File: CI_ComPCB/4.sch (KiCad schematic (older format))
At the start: 12 parts, among them IC301 TPS63020DSJR, J301 Connector_Conn_01x02_Male, J302 Connector_Conn_01x02_Male

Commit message: V1.1 Rough
Almost complete
needs silk screen annotations then will be ready to have printed
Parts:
- D301: symbol SamacSys_Parts:SS34 -> CI_ComPCB-rescue:SS34-SamacSys_Parts
- IC301: symbol SamacSys_Parts:TPS63020DSJR -> CI_ComPCB-rescue:TPS63020DSJR-SamacSys_Parts
- J301, J302: symbol CI_ComPCB-cache:Connector_Conn_01x02_Male -> CI_ComPCB-rescue:Connector_Conn_01x02_Male-CI_ComPCB-cache
- L301: symbol SamacSys_Parts:SPM4012T-1R0M-LR -> CI_ComPCB-rescue:SPM4012T-1R0M-LR-SamacSys_Parts
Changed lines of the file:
@@
 	6570 3680 6820 3680
 $Comp
-L SamacSys_Parts:TPS63020DSJR IC?
+L CI_ComPCB-rescue:TPS63020DSJR-SamacSys_Parts IC?
 U 1 1 61A532F4
 P 5770 4280
@@
 Buck_Converter_OUT
 $Comp
-L CI_ComPCB-cache:Connector_Conn_01x02_Male J301
+L CI_ComPCB-rescue:Connector_Conn_01x02_Male-CI_ComPCB-cache J301
 U 1 1 61294C10
 P 3410 3380
+AR Path="/61294C10" Ref="J301"  Part="1"
+AR Path="/61A31654/61294C10" Ref="J301"  Part="1"
 F 0 "J301" V 3472 3424 50  0000 L CNN
 F 1 "Connector_Conn_01x02_Male" V 3563 3424 50  0000 L CNN
@@
 $EndComp
 $Comp
-L CI_ComPCB-cache:Connector_Conn_01x02_Male J302
+L CI_ComPCB-rescue:Connector_Conn_01x02_Male-CI_ComPCB-cache J302
 U 1 1 61298A1D
 P 7470 3300
+AR Path="/61298A1D" Ref="J302"  Part="1"
+AR Path="/61A31654/61298A1D" Ref="J302"  Part="1"
 F 0 "J302" V 7532 3344 50  0000 L CNN
 F 1 "Connector_Conn_01x02_Male" V 7623 3344 50  0000 L CNN
@@
 $EndComp
 $Comp
-L SamacSys_Parts:SS34 D301
+L CI_ComPCB-rescue:SS34-SamacSys_Parts D301
 U 1 1 612A7837
 P 3450 3580
@@
 	4150 3580 4140 3580
 $Comp
-L SamacSys_Parts:SPM4012T-1R0M-LR L301
+L CI_ComPCB-rescue:SPM4012T-1R0M-LR-SamacSys_Parts L301
 U 1 1 612BD9BA
 P 5180 2700

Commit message: V1.1 Changed Diode for reprint
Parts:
- D301: footprint SamacSys_Parts:DIOM8059X256N -> digikey-footprints:DO-214AC
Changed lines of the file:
@@
 F 0 "D301" H 3850 3847 50  0000 C CNN
 F 1 "SS34" H 3850 3756 50  0000 C CNN
-F 2 "SamacSys_Parts:DIOM8059X256N" H 3950 3730 50  0001 L CNN
+F 2 "digikey-footprints:DO-214AC" H 3950 3730 50  0001 L CNN
 F 3 "https://componentsearchengine.com/Datasheets/2/SS34.pdf" H 3950 3630 50  0001 L CNN
 F 4 "ON Semi SS34 SMT Schottky Diode, 40V 3A, 2-Pin DO-214AB" H 3950 3530 50  0001 L CNN "Description"

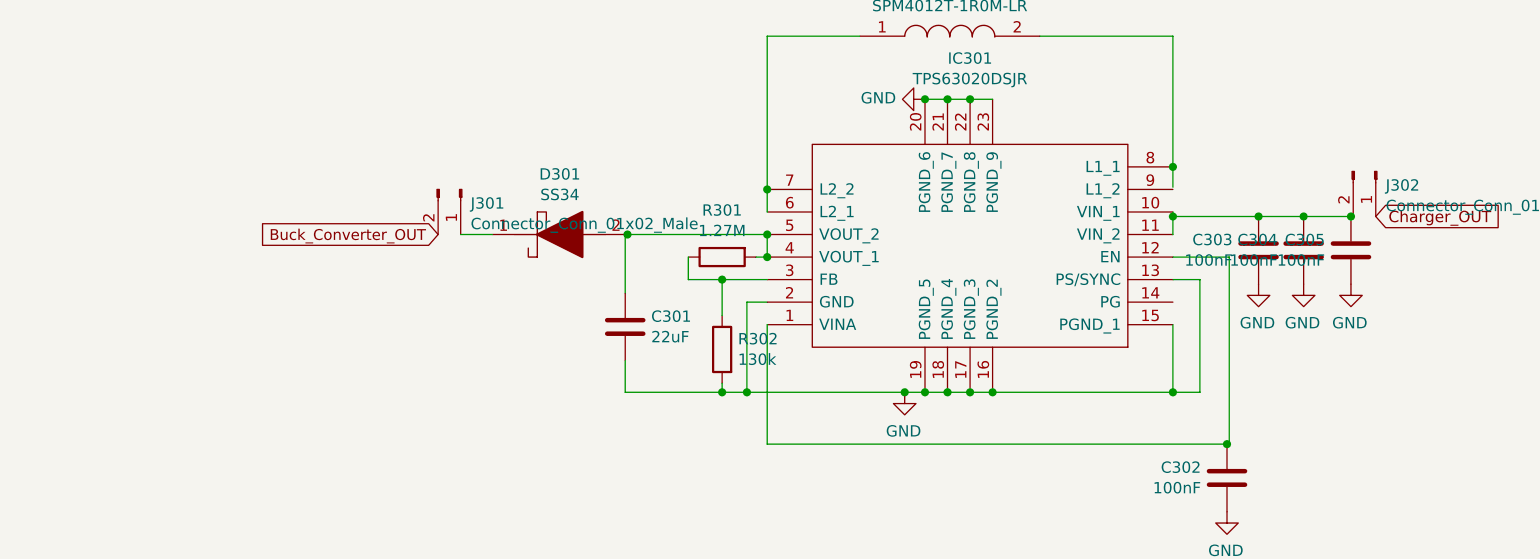
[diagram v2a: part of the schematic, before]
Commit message: converters debug
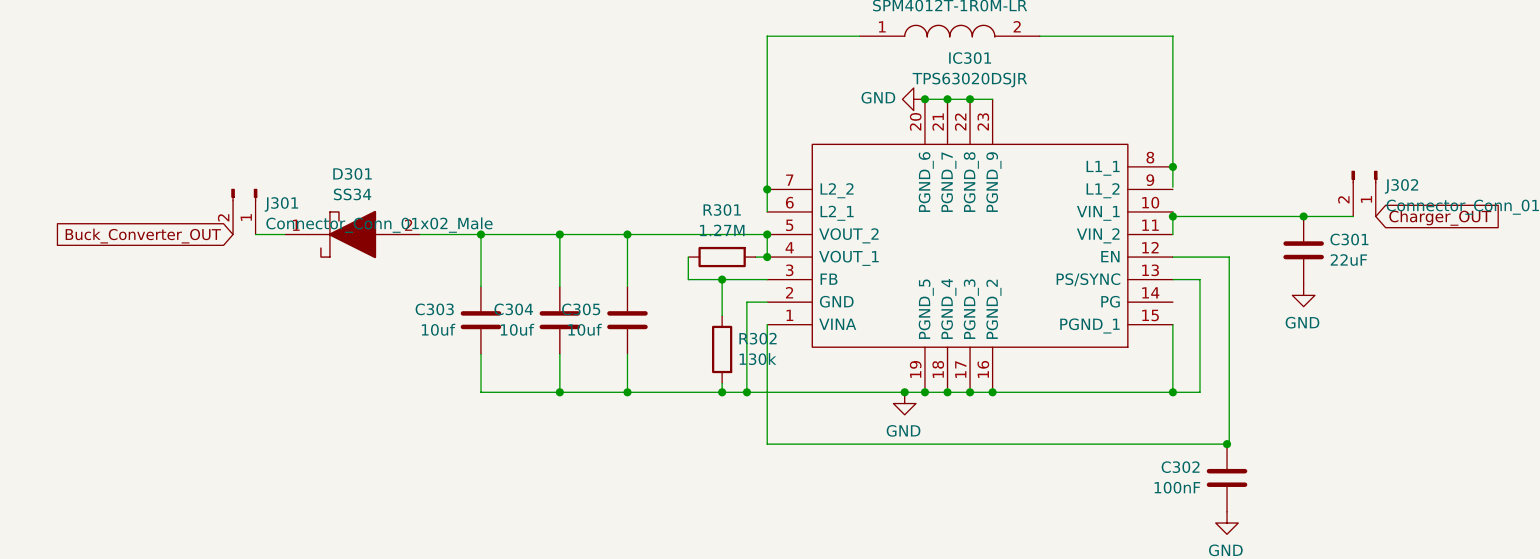
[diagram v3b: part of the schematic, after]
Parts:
- C303, C304, C305: value 100nF -> 10uf
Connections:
- net at IC301.10 (VIN_1), IC301.11 (VIN_2), J302.2 (Pin_2): now also C301.1; no longer C303.1, C304.1, C305.1
- net at D301.2, IC301.4 (VOUT_1), IC301.5 (VOUT_2)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: now also C303.1, C304.1, C305.1; no longer C301.1
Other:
- moved on the sheet: C301, C303, C304, C305, D301, J301
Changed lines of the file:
@@
 L Device:C C?
 U 1 1 61A53270
-P 4140 3990
+P 7150 3650
 AR Path="/61A53270" Ref="C?"  Part="1"
 AR Path="/61A31654/61A53270" Ref="C301"  Part="1"
-F 0 "C301" H 4025 4036 50  0000 R CNN
-F 1 "22uF" H 4025 3945 50  0000 R CNN
-F 2 "Capacitor_SMD:C_0805_2012Metric" H 4178 3840 50  0001 C CNN
-F 3 "~" H 4140 3990 50  0001 C CNN
-	1    4140 3990
-	-1   0    0    -1
-$EndComp
-Wire Wire Line
-	4770 3580 4150 3580
-Wire Wire Line
-	4140 3580 4140 3840
+F 0 "C301" H 7035 3696 50  0000 R CNN
+F 1 "22uF" H 7035 3605 50  0000 R CNN
+F 2 "Capacitor_SMD:C_0805_2012Metric" H 7188 3500 50  0001 C CNN
+F 3 "~" H 7150 3650 50  0001 C CNN
+	1    7150 3650
+	-1   0    0    -1
+$EndComp
 Wire Wire Line
 	5180 2700 4770 2700
@@
 	4570 4240 4570 4280
 Wire Wire Line
-	4570 4280 4140 4280
-Connection ~ 4570 4280
-Wire Wire Line
-	4140 4280 4140 4140
-Wire Wire Line
 	4770 4510 4770 3980
 Wire Wire Line
@@
 L Device:C C?
 U 1 1 61A532A2
-P 6950 3650
+P 3500 3960
 AR Path="/61A532A2" Ref="C?"  Part="1"
 AR Path="/61A31654/61A532A2" Ref="C303"  Part="1"
-F 0 "C303" H 7065 3696 50  0000 L CNN
-F 1 "100nF" H 7065 3605 50  0000 L CNN
-F 2 "Capacitor_SMD:C_0805_2012Metric" H 6988 3500 50  0001 C CNN
-F 3 "~" H 6950 3650 50  0001 C CNN
-	1    6950 3650
-	-1   0    0    -1
-$EndComp
-$Comp
-L power:GND #PWR?
-U 1 1 61A532A8
-P 6950 3800
-AR Path="/61A532A8" Ref="#PWR?"  Part="1"
-AR Path="/61A31654/61A532A8" Ref="#PWR0304"  Part="1"
-F 0 "#PWR0304" H 6950 3550 50  0001 C CNN
-F 1 "GND" H 6955 3627 50  0000 C CNN
-F 2 "" H 6950 3800 50  0001 C CNN
-F 3 "" H 6950 3800 50  0001 C CNN
-	1    6950 3800
-	-1   0    0    -1
-$EndComp
-Wire Wire Line
-	7370 3500 7360 3500
+F 0 "C303" H 3615 4006 50  0000 L CNN
+F 1 "10uf" H 3615 3915 50  0000 L CNN
+F 2 "Capacitor_SMD:C_0805_2012Metric" H 3538 3810 50  0001 C CNN
+F 3 "~" H 3500 3960 50  0001 C CNN
+	1    3500 3960
+	-1   0    0    -1
+$EndComp
 Text GLabel 7470 3500 2    50   Input ~ 0
 Charger_OUT
-Wire Wire Line
-	3410 3580 3550 3580
 Text Notes 7000 7110 0    50   ~ 0
 https://webench.ti.com/power-designer/switching-regulator/customize/6?noparams=0
@@
 L Device:C C?
 U 1 1 61A532B9
-P 7150 3650
+P 3850 3960
 AR Path="/61A532B9" Ref="C?"  Part="1"
 AR Path="/61A31654/61A532B9" Ref="C304"  Part="1"
-F 0 "C304" H 7265 3696 50  0000 L CNN
-F 1 "100nF" H 7265 3605 50  0000 L CNN
-F 2 "Capacitor_SMD:C_0805_2012Metric" H 7188 3500 50  0001 C CNN
-F 3 "~" H 7150 3650 50  0001 C CNN
-	1    7150 3650
+F 0 "C304" H 3965 4006 50  0000 L CNN
+F 1 "10uf" H 3965 3915 50  0000 L CNN
+F 2 "Capacitor_SMD:C_0805_2012Metric" H 3888 3810 50  0001 C CNN
+F 3 "~" H 3850 3960 50  0001 C CNN
+	1    3850 3960
 	-1   0    0    -1
 $EndComp
@@
 L Device:C C?
 U 1 1 61A532C5
-P 7360 3650
+P 4150 3960
 AR Path="/61A532C5" Ref="C?"  Part="1"
 AR Path="/61A31654/61A532C5" Ref="C305"  Part="1"
-F 0 "C305" H 7475 3696 50  0000 L CNN
-F 1 "100nF" H 7475 3605 50  0000 L CNN
-F 2 "Capacitor_SMD:C_0805_2012Metric" H 7398 3500 50  0001 C CNN
-F 3 "~" H 7360 3650 50  0001 C CNN
-	1    7360 3650
-	-1   0    0    -1
-$EndComp
-$Comp
-L power:GND #PWR?
-U 1 1 61A532CB
-P 7360 3800
-AR Path="/61A532CB" Ref="#PWR?"  Part="1"
-AR Path="/61A31654/61A532CB" Ref="#PWR0306"  Part="1"
-F 0 "#PWR0306" H 7360 3550 50  0001 C CNN
-F 1 "GND" H 7365 3627 50  0000 C CNN
-F 2 "" H 7360 3800 50  0001 C CNN
-F 3 "" H 7360 3800 50  0001 C CNN
-	1    7360 3800
-	-1   0    0    -1
-$EndComp
-Connection ~ 7150 3500
-Connection ~ 7360 3500
-Wire Wire Line
-	7360 3500 7150 3500
-Wire Wire Line
-	6950 3500 7150 3500
+F 0 "C305" H 4265 4006 50  0000 L CNN
+F 1 "10uf" H 4265 3915 50  0000 L CNN
+F 2 "Capacitor_SMD:C_0805_2012Metric" H 4188 3810 50  0001 C CNN
+F 3 "~" H 4150 3960 50  0001 C CNN
+	1    4150 3960
+	-1   0    0    -1
+$EndComp
 Connection ~ 6570 3280
 Connection ~ 5670 4280
@@
 Wire Wire Line
 	6570 3480 6570 3500
-Wire Wire Line
-	6950 3500 6570 3500
-Connection ~ 6950 3500
 Connection ~ 6570 3500
 Wire Wire Line
 	6570 3500 6570 3580
-Text GLabel 3310 3580 0    48   Input ~ 0
+Text GLabel 2400 3580 0    48   Input ~ 0
 Buck_Converter_OUT
 $Comp
 L CI_ComPCB-rescue:Connector_Conn_01x02_Male-CI_ComPCB-cache J301
 U 1 1 61294C10
-P 3410 3380
+P 2500 3380
 AR Path="/61294C10" Ref="J301"  Part="1"
 AR Path="/61A31654/61294C10" Ref="J301"  Part="1"
-F 0 "J301" V 3472 3424 50  0000 L CNN
-F 1 "Connector_Conn_01x02_Male" V 3563 3424 50  0000 L CNN
-F 2 "Connector_PinHeader_2.54mm:PinHeader_1x02_P2.54mm_Vertical" H 3410 3380 50  0001 C CNN
-F 3 "" H 3410 3380 50  0001 C CNN
-	1    3410 3380
+F 0 "J301" V 2562 3424 50  0000 L CNN
+F 1 "Connector_Conn_01x02_Male" V 2653 3424 50  0000 L CNN
+F 2 "Connector_PinHeader_2.54mm:PinHeader_1x02_P2.54mm_Vertical" H 2500 3380 50  0001 C CNN
+F 3 "" H 2500 3380 50  0001 C CNN
+	1    2500 3380
 	0    1    1    0
 $EndComp
@@
 	0    1    1    0
 $EndComp
-$Comp
-L CI_ComPCB-rescue:SS34-SamacSys_Parts D301
-U 1 1 612A7837
-P 3450 3580
-F 0 "D301" H 3850 3847 50  0000 C CNN
-F 1 "SS34" H 3850 3756 50  0000 C CNN
-F 2 "digikey-footprints:DO-214AC" H 3950 3730 50  0001 L CNN
-F 3 "https://componentsearchengine.com/Datasheets/2/SS34.pdf" H 3950 3630 50  0001 L CNN
-F 4 "ON Semi SS34 SMT Schottky Diode, 40V 3A, 2-Pin DO-214AB" H 3950 3530 50  0001 L CNN "Description"
-F 5 "2.56" H 3950 3430 50  0001 L CNN "Height"
-F 6 "512-SS34" H 3950 3330 50  0001 L CNN "Mouser Part Number"
-F 7 "https://www.mouser.co.uk/ProductDetail/ON-Semiconductor-Fairchild/SS34?qs=2ONuHmP%2FXzb3ub11UdFfdQ%3D%3D" H 3950 3230 50  0001 L CNN "Mouser Price/Stock"
-F 8 "ON Semiconductor" H 3950 3130 50  0001 L CNN "Manufacturer_Name"
-F 9 "SS34" H 3950 3030 50  0001 L CNN "Manufacturer_Part_Number"
-	1    3450 3580
-	1    0    0    -1
-$EndComp
-Connection ~ 4150 3580
-Wire Wire Line
-	4150 3580 4140 3580
 $Comp
 L CI_ComPCB-rescue:SPM4012T-1R0M-LR-SamacSys_Parts L301
@@
 Wire Wire Line
 	5980 2700 6570 2700
+Wire Wire Line
+	6570 3500 7150 3500
+Wire Wire Line
+	3500 4280 3500 4110
+Connection ~ 4570 4280
+Wire Wire Line
+	3850 4110 3850 4280
+Connection ~ 3850 4280
+Wire Wire Line
+	3850 4280 3500 4280
+Wire Wire Line
+	4570 4280 4150 4280
+Wire Wire Line
+	4150 4110 4150 4280
+Connection ~ 4150 4280
+Wire Wire Line
+	4150 4280 3850 4280
+Wire Wire Line
+	3500 3810 3500 3580
+Connection ~ 3500 3580
+Wire Wire Line
+	3850 3810 3850 3580
+Connection ~ 3850 3580
+Wire Wire Line
+	3850 3580 3500 3580
+Wire Wire Line
+	4770 3580 4150 3580
+Wire Wire Line
+	4150 3810 4150 3580
+Connection ~ 4150 3580
+Wire Wire Line
+	4150 3580 3850 3580
+Connection ~ 7150 3500
+Wire Wire Line
+	7150 3500 7370 3500
+Wire Wire Line
+	3230 3580 3500 3580
+$Comp
+L CI_ComPCB-rescue:SS34-SamacSys_Parts D301
+U 1 1 612A7837
+P 2530 3580
+F 0 "D301" H 2930 3847 50  0000 C CNN
+F 1 "SS34" H 2930 3756 50  0000 C CNN
+F 2 "digikey-footprints:DO-214AC" H 3030 3730 50  0001 L CNN
+F 3 "https://componentsearchengine.com/Datasheets/2/SS34.pdf" H 3030 3630 50  0001 L CNN
+F 4 "ON Semi SS34 SMT Schottky Diode, 40V 3A, 2-Pin DO-214AB" H 3030 3530 50  0001 L CNN "Description"
+F 5 "2.56" H 3030 3430 50  0001 L CNN "Height"
+F 6 "512-SS34" H 3030 3330 50  0001 L CNN "Mouser Part Number"
+F 7 "https://www.mouser.co.uk/ProductDetail/ON-Semiconductor-Fairchild/SS34?qs=2ONuHmP%2FXzb3ub11UdFfdQ%3D%3D" H 3030 3230 50  0001 L CNN "Mouser Price/Stock"
+F 8 "ON Semiconductor" H 3030 3130 50  0001 L CNN "Manufacturer_Name"
+F 9 "SS34" H 3030 3030 50  0001 L CNN "Manufacturer_Part_Number"
+	1    2530 3580
+	1    0    0    -1
+$EndComp
+Wire Wire Line
+	2630 3580 2500 3580
 $EndSCHEMATC
